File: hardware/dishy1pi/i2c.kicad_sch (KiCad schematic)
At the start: 19 parts, among them CN3 KF2EDGR-2.54-4P, CN4 KF2EDGR-2.54-4P, U6 LTC4311ISC6#TRPBF, U7 ISO1540DR, U8 LM75BIMX-5/NOPB

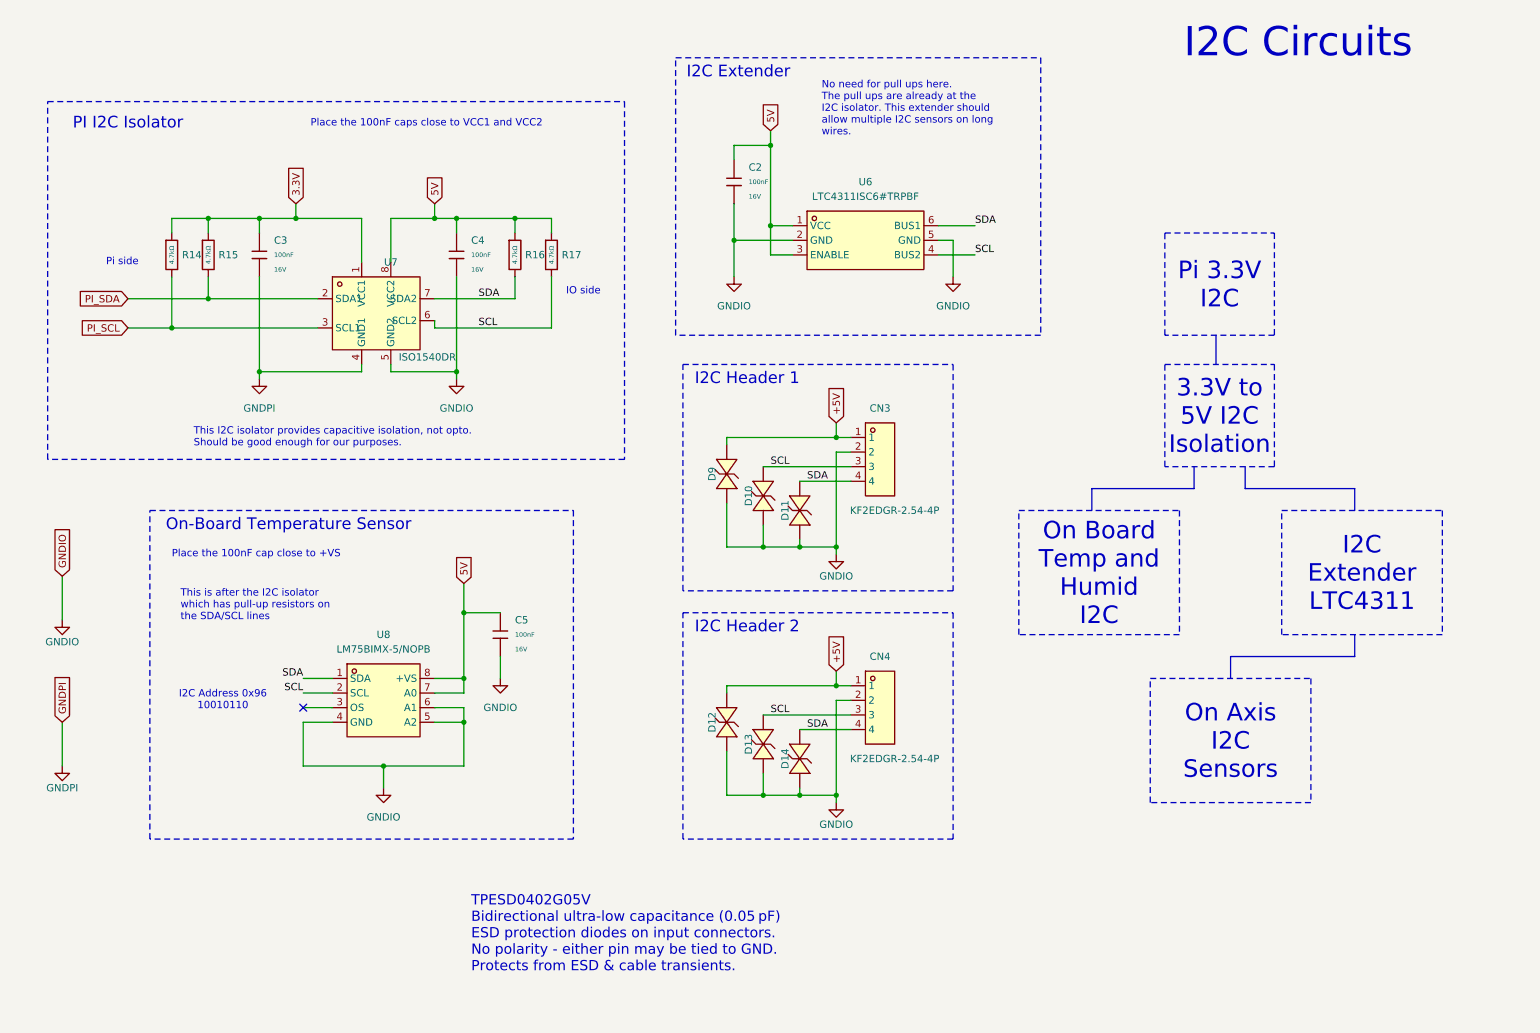
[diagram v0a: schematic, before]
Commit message: Pushed latest parts lib
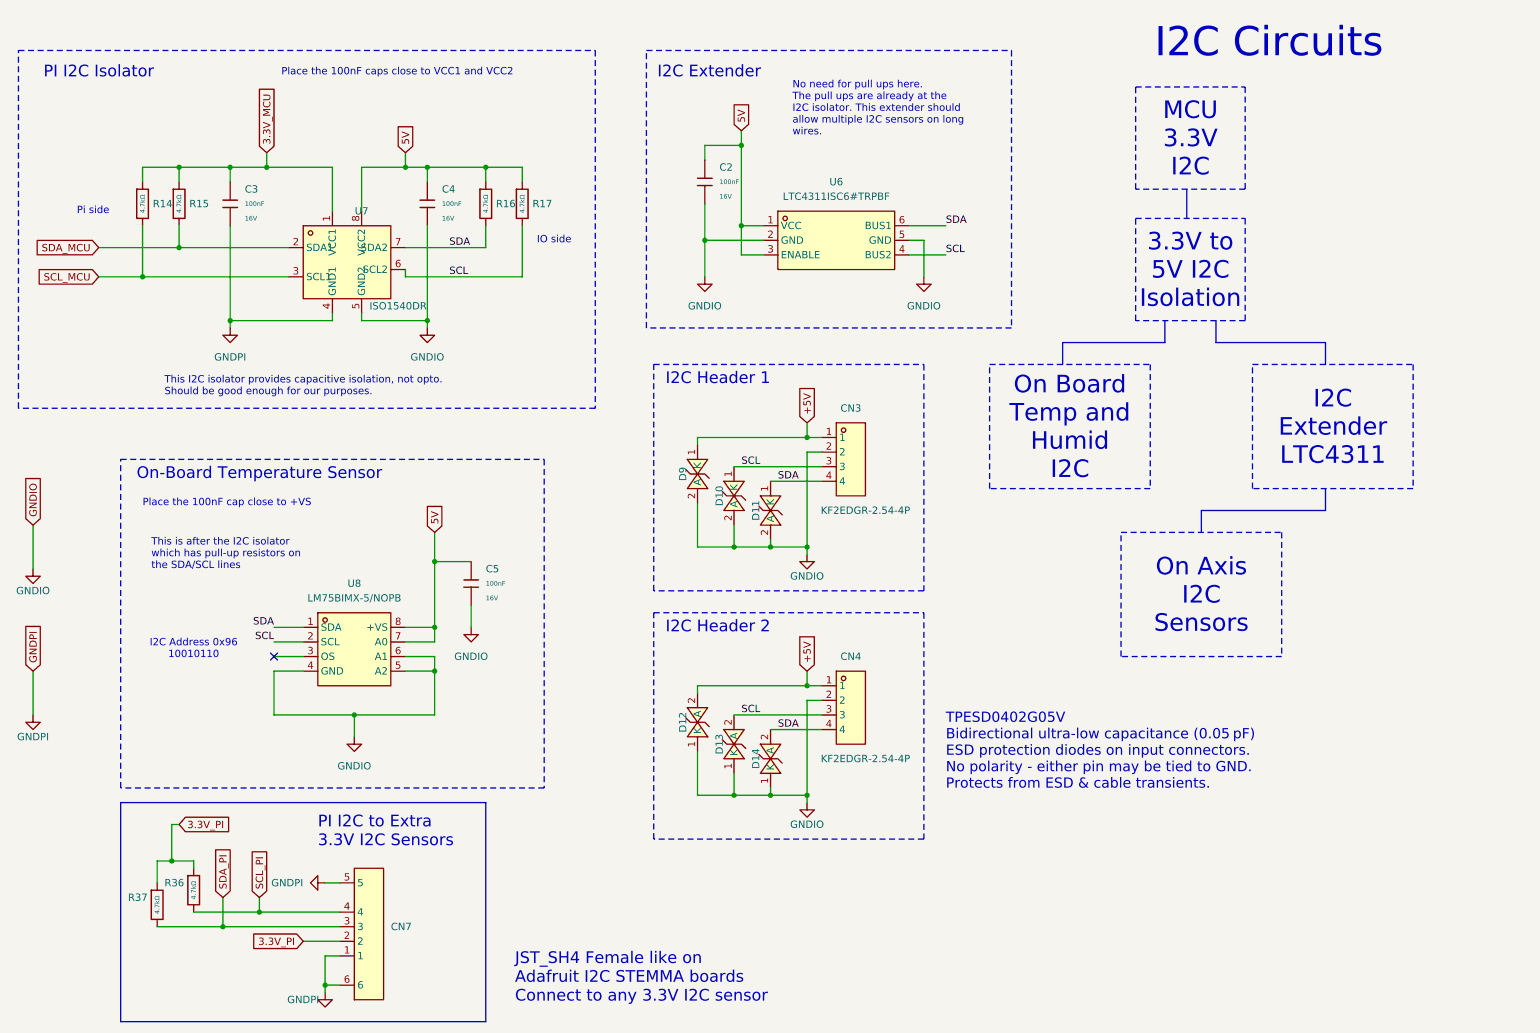
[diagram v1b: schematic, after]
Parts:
- added CN7: SM04B-SRSS-TB (LF)(SN), MyParts:CONN-SMD_4P-P1.00_SM04B-SRSS-TB-LF-SN, symbol MyParts:SM04B-SRSS-TB(LF)(SN)
- added R36, R37: 4.7kΩ, PCM_JLCPCB:R_0402, symbol PCM_JLCPCB-Resistors:0402,4.7kΩ
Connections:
- net GNDPI: now also CN7.1, CN7.5, CN7.6
- net 3.3V renamed 3.3V_MCU
- net PI_SCL renamed SCL_MCU
- net PI_SDA renamed SDA_MCU
- new net 3.3V_PI: CN7.2, R36.1, R37.1
- new net SCL_PI: CN7.4, R36.2
- new net SDA_PI: CN7.3, R37.2
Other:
- note added: "JST_SH4 Female like on Adafruit I2C STEMMA boards Connect to any 3.3V I2C sensor"
- note added: "PI I2C to Extra 3.3V I2C Sensors"
- moved on the sheet: C2, C3, C4, C5, CN3, CN4, R14, R15, R16, R17, U6, U7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
